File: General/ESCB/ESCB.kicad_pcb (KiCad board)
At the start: 2 copper layers, 35.8 x 17.5 mm, 3 parts, among them J1 Power_Signal, J2 Motor, U1 BESC

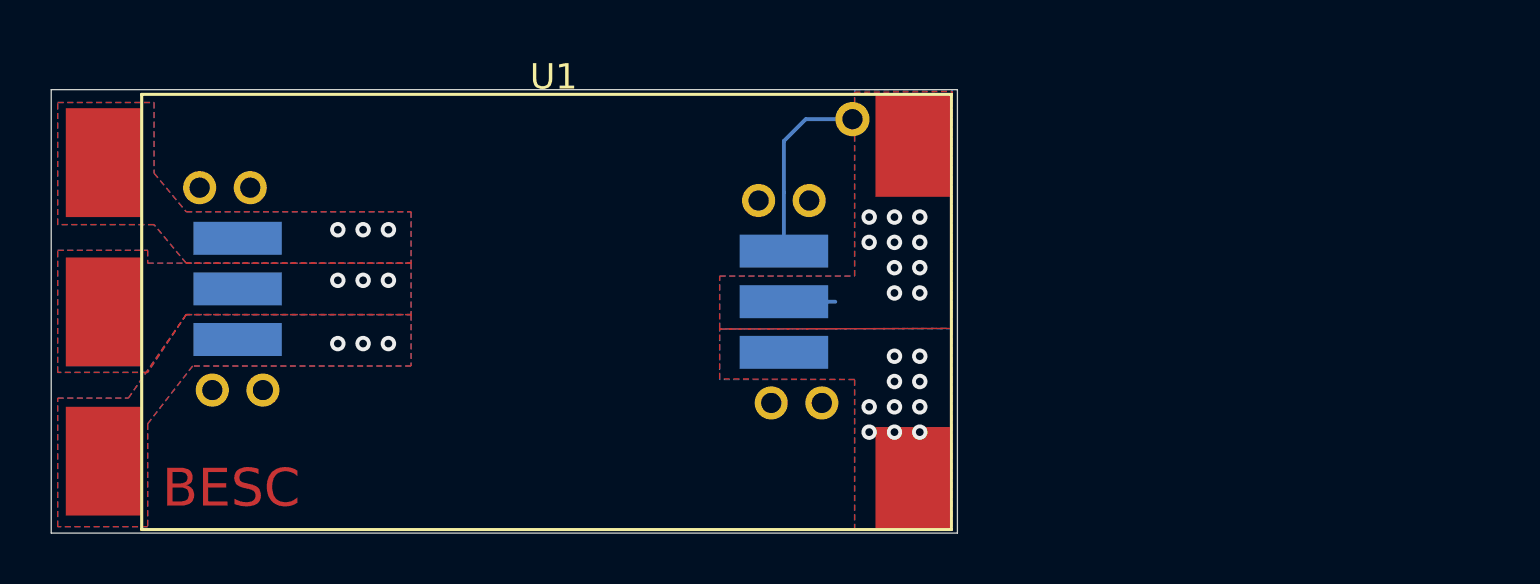
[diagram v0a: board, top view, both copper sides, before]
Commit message: Update ESCB.kicad_pcb
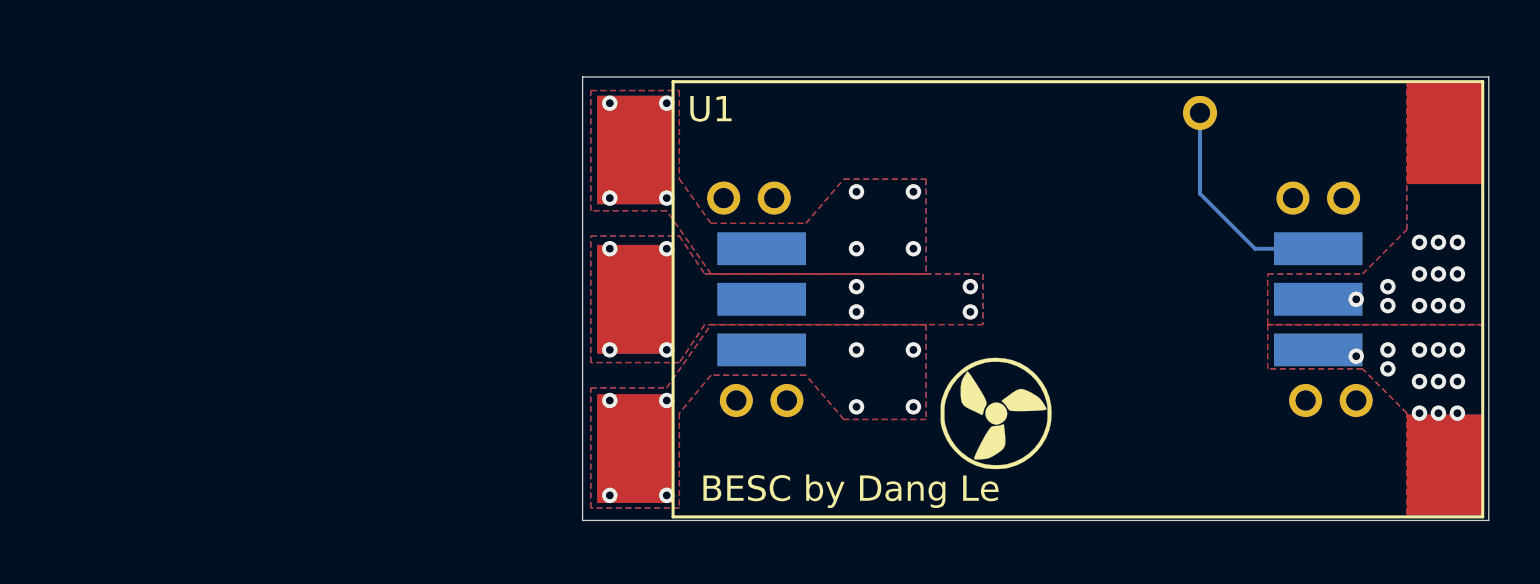
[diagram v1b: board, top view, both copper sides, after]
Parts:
- added G***: LOGO, extraparts:auv_logo, F.Cu at (159.5, 105.8)
- moved J1 21.1 mm to (172.2, 101.2)
- moved U1 21.0 mm to (162.8, 101.2)
- moved J2 20.7 mm to (150.2, 101.2)
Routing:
- net VCC: track 2.54 -> 0.00 mm, vias 10 -> 12
- net Net-(J1-Pad3): track 7.61 -> 8.96 mm
- net Net-(J2-Pad3): vias 3 -> 8
- net Net-(J2-Pad2): vias 3 -> 8
- net Net-(J2-Pad1): vias 3 -> 8
- net GND: vias 10 -> 12
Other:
- board text added: "BESC by Dang Le"
- board text removed: "BESC"
